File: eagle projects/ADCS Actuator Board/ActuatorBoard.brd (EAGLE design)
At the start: 91 x 91 mm, 259 parts, among them J4 OSTVN08A150, J5 OSTVN08A150, J6 OSTVN08A150, U10 TVS991, U11 BD6210F-E2, U12 ADS7841E_2K5, U13 ADS7841E_2K5, U15 TLV9051IDCKR, U16 BD6210F-E2, U17 DRV10970_MOTOR_DRIVERDRV10970, U18 DRV10970_MOTOR_DRIVERDRV10970, U19 TLV9051IDCKR, U20 DRV10970_MOTOR_DRIVERDRV10970, U21 TLV9051IDCKR, U22 BD6210F-E2, U23 TLV9051IDCKR, U24 TLV9051IDCKR, U25 ADS7841E_2K5, U26 TLV9051IDCKR, U27 ADS7841E_2K5, U28 TLV9051IDCKR, U29 TLV9051IDCKR, U30 TLV9051IDCKR, U31 TLV9051IDCKR, U32 TLV9051IDCKR, U4 ADS7841E_2K5, U6 TLV9051IDCKR, U7 TVS991, U8 TVS991, U9 ADS7841E_2K5

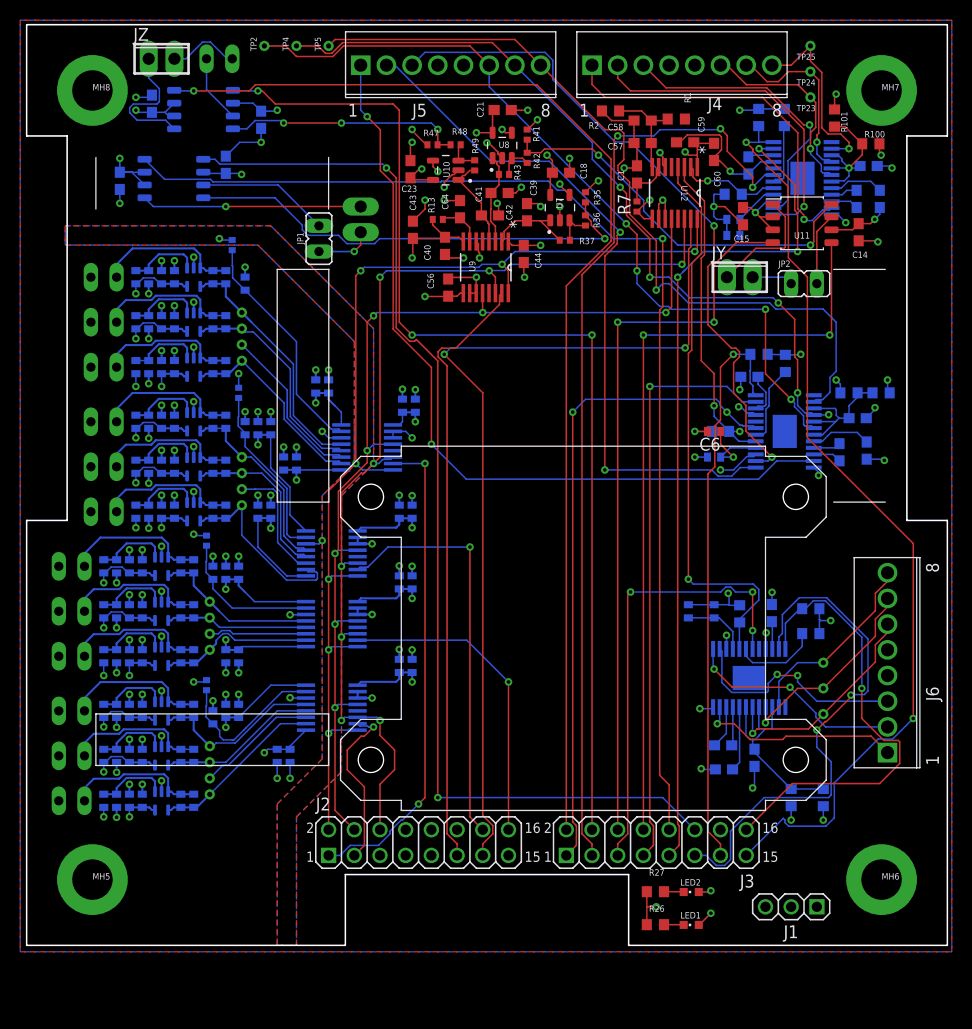
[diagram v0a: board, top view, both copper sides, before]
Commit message: moved a bunch of digital shit around (work in progress). going to sleep now
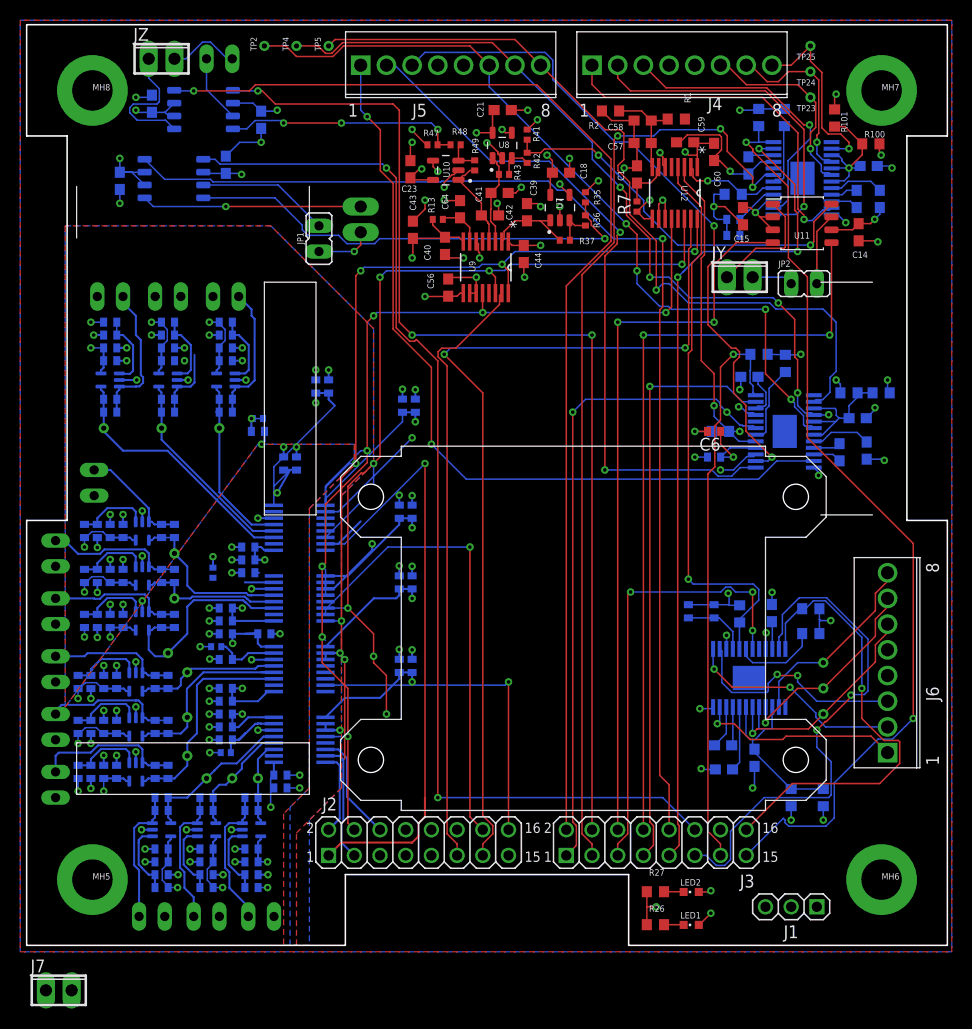
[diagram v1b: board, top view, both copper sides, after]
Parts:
- removed TP1, TP13, TP17, TP9: TESTPOINT, my_library:TP_P76H50
- added J7: (no value), my_library:2POL254
- moved D13 21.9 mm to (23.2, 2.86), turned to 90 degrees
- moved D15 21.8 mm to (12.4, 2.86), turned to 90 degrees
- moved D14 20.7 mm to (17.8, 2.86), turned to 90 degrees
- moved R69 18.4 mm to (13.3, 5.71), turned to 180 degrees
- moved R4 18.0 mm to (18.4, 36.8)
- moved R6 17.3 mm to (22.9, 52.1), turned to 180 degrees
- moved R63 16.9 mm to (22.2, 5.71), turned to 180 degrees
- moved R68 16.8 mm to (13.3, 6.99), turned to 0 degrees
- moved R66 16.5 mm to (17.8, 5.71), turned to 180 degrees
- moved TP10 16.3 mm to (14.0, 28.9)
- moved C113 15.3 mm to (13.3, 8.26), turned to 0 degrees
- moved R62 15.2 mm to (22.2, 6.99), turned to 0 degrees
- moved TP3 15.2 mm to (7.62, 51.1), turned to 90 degrees
- moved R65 14.7 mm to (17.8, 6.99), turned to 0 degrees
- moved C81 14.7 mm to (22.9, 50.8), turned to 180 degrees
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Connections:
- removed net N$37: TP1.1, U4.3
- removed net N$48: TP9.1, U13.3
- removed net N$59: TP13.1, U25.3
- removed net N$67: TP17.1, U27.3
- net X+_0_DEGREES: now also U25.3; no longer U25.2
- net X-_0_DEGREES: now also U13.3; no longer U13.2
- net Y+_0_DEGREES: now also U27.3; no longer U27.2
- net Y-_0_DEGREES: now also U4.3; no longer U4.2
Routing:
- net N$24: track 22.8 -> 1.95 mm
- net !CS!_SUN_Y-: track 48.2 -> 64.3 mm, vias 2 -> 1
- net N$37: track 16.1 -> 0.00 mm
- net +3V3: track 227.1 -> 243.0 mm
- net GND: track 216.0 -> 230.7 mm
- net N$22: track 17.5 -> 3.34 mm
- net N$48: track 12.2 -> 0.00 mm
- net N$67: track 12.0 -> 0.00 mm
- net N$59: track 9.78 -> 0.00 mm
- net Y+_0_DEGREES: track 17.2 -> 8.73 mm
- net N$25: track 15.8 -> 7.45 mm
- net N$4: track 14.5 -> 6.35 mm
- net N$33: track 14.2 -> 7.24 mm
- net Y-_240_DEGREES: track 24.3 -> 17.7 mm
- net UCB0_SPI_MISO: track 103.5 -> 109.7 mm
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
